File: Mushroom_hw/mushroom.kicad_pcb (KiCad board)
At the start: 2 copper layers, 49.2 x 83.8 mm, 129 parts, among them Q1 LED_RGB_WS2812B, Q2 LED_RGB, Q3 LED_RGB_WS2812B, Q4 LED_RGB, Q5 LED_RGB, Q6 LED_RGB_WS2812B, SW1 SWITCH_H

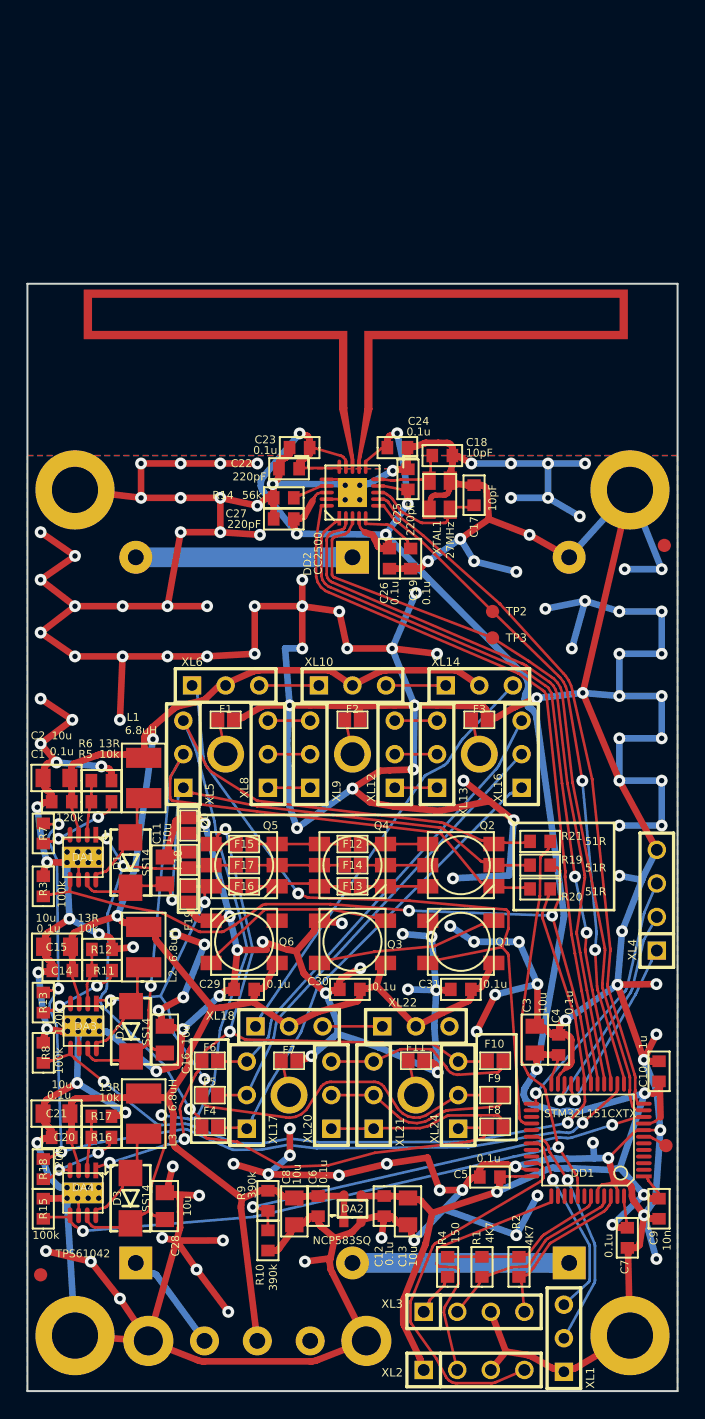
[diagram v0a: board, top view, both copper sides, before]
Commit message: + Component placement done
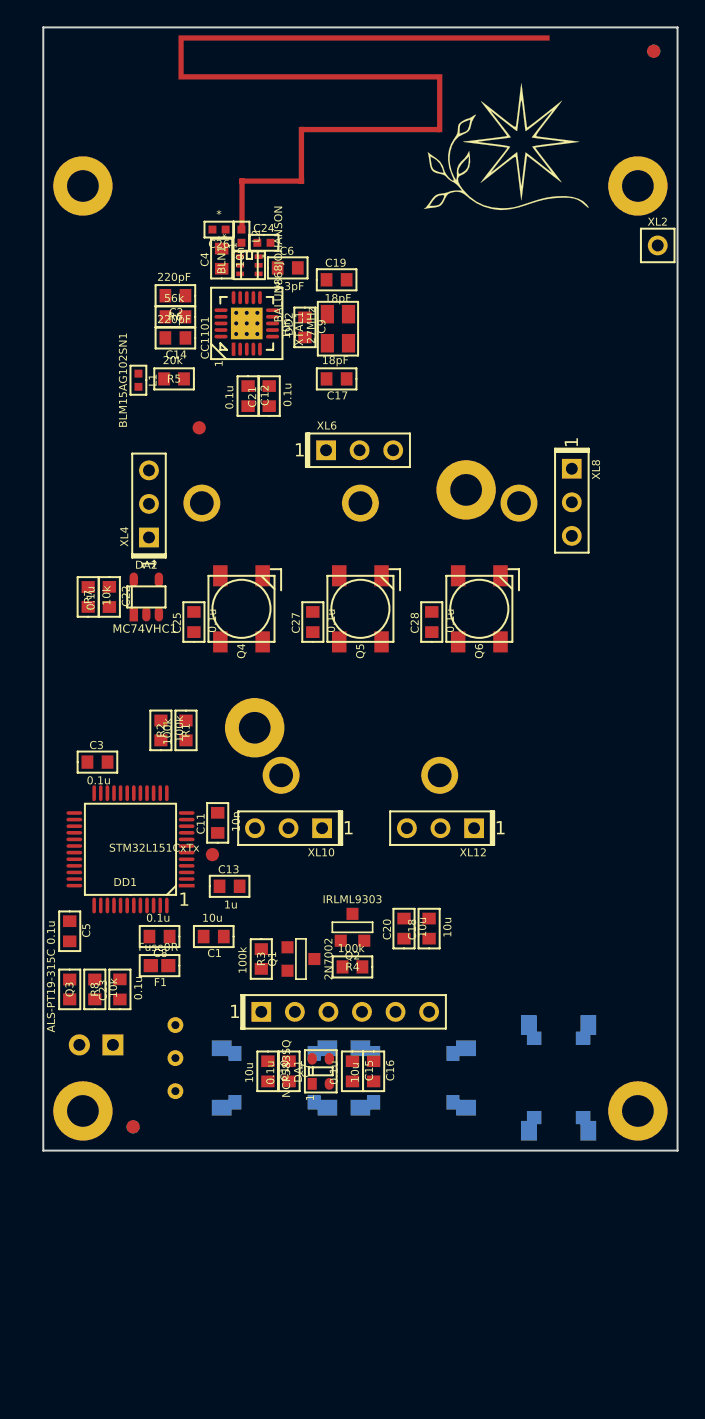
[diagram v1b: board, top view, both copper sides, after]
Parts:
- removed B1, B2, B3: BAT, BAT_AA
- removed C29, C30, C31: 0.1u, CAP_0603
- removed D1, D2, D3: SS14, DIODE_SMA_DO214AC
- removed DA3, DA4: TPS61042, DRB8
- removed F10, F11, F12, F13, F14, F15, F16, F17, F18, F19, F2, F20, F3, F4, F5, F6, F7, F8, F9: FUSE0R, SMD0603_FUSE
- removed L3: 6.8uH, IND_1210
- removed R10, R9: 390k, RES_0603
- removed R11, R16: 10k, RES_0603
- removed R12, R17: 13R, RES_0603
- removed R13, R18: 120k, RES_0603
- removed R14: 56k, RES_0603
- removed R15: 100k, RES_0603
- removed R19, R20, R21: 51R, RES_0603
- removed TP3: TESTPOINT, TESTPOINT_1MM
- removed XL14, XL16, XL17, XL18, XL20, XL21, XL22, XL24: CONN_3, SIL-3
- removed XL15, XL19, XL23: CONN_1, SIL1_ROUND_1MM8
- added BLN1: BALUN868JOHANSON, Radio:BALUN_JOHANSON868, F.Cu at (219.6, 130.0)
- added HOLE5: HOLE_METALLED, PCB:Hole2d4_out4d5mm, F.Cu at (249.0, 194.0)
- added HOLE6: HOLE_METALLED, PCB:Hole2d4_out4d5mm, F.Cu at (249.0, 124.0)
- added Logo1: Logo, Pictures:Ostranna_12d7_10d1, F.Cu at (239.0, 121.0)
- added RP3: REFPOINT, PCB:REF_POINT_1MM, B.Cu at (210.8, 195.2)
- added RP4: REFPOINT, PCB:REF_POINT_1MM, B.Cu at (250.2, 113.8)
- added SW2: BUTTON, BtnsSwitches:BTN_6x6_4x4, B.Cu at (243.0, 191.5)
- added SW3: BUTTON, BtnsSwitches:BTN_6x6_4x4, B.Cu at (221.5, 191.5)
- added SW4: BUTTON, BtnsSwitches:BTN_6x6_4x4, B.Cu at (232.0, 191.5)
- ANT1: value ANT_PCB_NOCNTR -> ANT_PCB_MONO; footprint ANT_FOLDED_DIPOLE2 -> Radio:ANT_868_ARMLETG
- C1, C20: value 0.1u -> 10u; footprint CAP_0603 -> Capacitors:CAP_0603
- C10: value 1u -> 10u; footprint CAP_0603 -> Capacitors:CAP_0603
- C11: value 10u -> 10n; footprint CAP_0805 -> Capacitors:CAP_0603
- C12, C23, C5, C7, C9: footprint CAP_0603 -> Capacitors:CAP_0603
- C13: value 10u -> 1u; footprint CAP_0805 -> Capacitors:CAP_0603
- C14: value 0.1u -> 220pF; footprint CAP_0603 -> Capacitors:CAP_0603
- C15, C21, C28, C3, C8: value 10u -> 0.1u; footprint CAP_0805 -> Capacitors:CAP_0603
- C16: footprint CAP_0805 -> Capacitors:CAP_0603
- C17: value 10pF -> 18pF; footprint CAP_0603 -> Capacitors:CAP_0603
- C18: value 10pF -> 10u; footprint CAP_0603 -> Capacitors:CAP_0603
- C19: value 0.1u -> 18pF; footprint CAP_0603 -> Capacitors:CAP_0603
- C2: value 10u -> 220pF; footprint CAP_0805 -> Capacitors:CAP_0603
- C22, C25, C27: value 220pF -> 0.1u; footprint CAP_0603 -> Capacitors:CAP_0603
- C24, C26: value 0.1u -> *; footprint CAP_0603 -> Capacitors:CAP_0402
- C4: value 0.1u -> 10n; footprint CAP_0603 -> Capacitors:CAP_0603
- C6: value 0.1u -> 3.3pF; footprint CAP_0603 -> Capacitors:CAP_0603
- DA1: value TPS61042 -> NCP583SQ; footprint DRB8 -> SOT:SC82AB
- DA2: value NCP583SQ -> MC74VHC1; footprint SC82AB -> SOT:SOT23-5
- DD1: value STM32L151CXTX -> STM32L151CxTx; footprint LQFP48 -> LQFP_TQFP:LQFP48
- DD2: value CC2500 -> CC1101; footprint QFN20 -> QFN_DFN:QFN20
- F1: value FUSE0R -> Fuse0R; footprint SMD0603_FUSE -> Resistors:RES_0603_FUSE
- HOLE1, HOLE2, HOLE3, HOLE4: footprint Hole3_5_out6mm -> PCB:Hole2d4_out4d5mm
- L1: value 6.8uH -> BLM15AG102SN1; footprint IND_1210 -> Inductors:IND_0402
- L2: value 6.8uH -> *; footprint IND_1210 -> Inductors:IND_0402
- Q1: value LED_RGB_WS2812B -> 2N7002; footprint LED_WS2812B -> SOT:SOT23-3
- Q2: value LED_RGB -> IRLML9303; footprint LED_HH5050_RGB -> SOT:SOT23-3
- Q3: value LED_RGB_WS2812B -> ALS-PT19-315C; footprint LED_WS2812B -> Resistors:RES_0603
- Q4, Q5: value LED_RGB -> LED_RGB_WS2812B; footprint LED_HH5050_RGB -> LEDs:LED_WS2812B
- Q6: footprint LED_WS2812B -> LEDs:LED_WS2812B
- R1, R2: value 4K7 -> 100k; footprint RES_0603 -> Resistors:RES_0603
- R3: footprint RES_0603 -> Resistors:RES_0603
- R4: value 150 -> 100k; footprint RES_0603 -> Resistors:RES_0603
- R5: value 10k -> 20k; footprint RES_0603 -> Resistors:RES_0603
- R6: value 13R -> 56k; footprint RES_0603 -> Resistors:RES_0603
- R7: value 120k -> 10k; footprint RES_0603 -> Resistors:RES_0603
- R8: value 100k -> 10k; footprint RES_0603 -> Resistors:RES_0603
- RP1, RP2: footprint REF_POINT_1MM -> PCB:REF_POINT_1MM
- SW1: value SWITCH_H -> SWITCH; footprint SWITCH_SS9 -> BtnsSwitches:SW_SS-1P2T
- TP1, TP2: footprint TESTPOINT_1MM -> PCB:TESTPOINT_1MM
- XL1: value CONN_3 -> CONN_6; footprint SIL-3 -> Connectors:PLS-6; moved to B.Cu
- XL10, XL12, XL6, XL8: footprint SIL-3 -> Connectors:PLS-3
- XL11, XL7: footprint SIL1_ROUND_1MM8 -> Connectors:SIL1_ROUND_1MM8
- XL13, XL5, XL9: value CONN_3 -> CONN_1; footprint SIL-3 -> Connectors:SIL1_ROUND_1MM8
- XL2: value ST_SWD -> CONN_1; footprint SIL-4 -> Connectors:PLS-1Rnd
- XL3: value CONN_4 -> CONN_2; footprint SIL-4 -> Connectors:W02_Pitch_2d54; moved to B.Cu
- XL4: value CONN_4 -> CONN_3; footprint SIL-4 -> Connectors:PLS-3
- XTAL1: footprint CRYSTAL_03225C4 -> Quartz:03225C4
- moved RP1 103.6 mm to (250.2, 113.8)
- moved XL2 86.2 mm to (250.5, 128.5)
- moved C9 71.9 mm to (223.8, 134.7)
- moved C6 71.0 mm to (222.5, 130.2), turned to 0 degrees
- moved C4 64.7 mm to (217.5, 129.5)
- moved C12 62.2 mm to (219.5, 139.9)
- moved RP2 59.6 mm to (210.8, 195.2)
- moved C21 56.6 mm to (221.1, 139.9), turned to 90 degrees
- moved L2 54.3 mm to (219.0, 127.8), turned to 270 degrees
- moved HOLE2 54.1 mm to (220.0, 165.0)
- moved DA2 48.9 mm to (211.8, 155.1), turned to 0 degrees
- moved R2 48.8 mm to (212.9, 165.2)
- moved C14 48.6 mm to (214.0, 135.5)
- moved C28 48.6 mm to (233.4, 157.0)
- moved HOLE4 47.4 mm to (207.0, 124.0)
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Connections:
- ANT1 pad 1: /Ant -> /ANT2
- C1 pad 1: +BATT -> GND
- C1 pad 2: GND -> +3.3V
- C10 pad 1: +3.3V -> +BATT
- C11 pad 1: /RED_P -> +3.3V
- C12 pad 1: +3.3V -> VCC
- C14 pad 1: +BATT -> VCC
- C15 pad 1: +BATT -> +3.3V
- C16 pad 1: /GREEN_P -> +3.3V
- C18 pad 1: N-000005 -> GND
- C18 pad 2: GND -> PwrUnst
- C19 pad 1: N-0000010 -> Net-(C19-Pad1)
- C2 pad 1: +BATT -> VCC
- C20 pad 1: +BATT -> GND
- C20 pad 2: GND -> PwrUnst
- C21 pad 1: +BATT -> GND
- C21 pad 2: GND -> Net-(C21-Pad2)
- C22 pad 1: +3.3V -> PwrUnst
- C23 pad 1: +3.3V -> /ADC_LUM
- C24 pad 1: +3.3V -> /ANT1
- C25 pad 1: +3.3V -> PwrUnst
- C26 pad 1: +3.3V -> /ANT2
- C27 pad 1: +3.3V -> PwrUnst
- C28 pad 1: /BLUE_P -> PwrUnst
- C4 pad 1: +3.3V -> VCC
- C6 pad 1: +BATT -> VCC
- C7 pad 1: +3.3V -> +BATT
- C8 pad 1: +BATT -> +3.3V
- C9 pad 1: +3.3V -> VCC
- DA1 pad 1: /RED_N -> +BATT
- DA1 pad 2: N-000007 -> GND
- DA1 pad 3: +BATT -> +3.3V
- DA1 pad 4: N-000006 -> +BATT
- DA2 pad 1: +BATT -> Net-(DA2-Pad1)
- DA2 pad 2: GND -> /WS_CTRL
- DA2 pad 3: +3.3V -> GND
- DA2 pad 4: +BATT -> /DIN0
- DD1 pad 10: N-000008 -> /BTN1
- DD1 pad 11: /CC_GDO2 -> /BTN2
- DD1 pad 12: /CC_CS -> /ADC_BATTERY
- DD1 pad 14: /BRIGHTNESS -> /CC_CS
- DD1 pad 18: /RED_PWM -> /ADC_LUM
- DD1 pad 19: /GREEN_PWM -> /MEAS_LUM
- DD1 pad 21: N-0000032 -> (no net)
- DD1 pad 22: N-0000033 -> (no net)
- DD1 pad 25: N-0000031 -> (no net)
- DD1 pad 27: (no net) -> /PWR_EN
- DD1 pad 28: /DIN0 -> /WS_CTRL
- DD1 pad 29: (no net) -> /BTN3
- DD1 pad 41: /BLUE_PWM -> (no net)
- DD1 pad 43: /PeriphPwr -> /NO_RADIO
- DD1 pad 45: /P_SCL -> (no net)
- DD1 pad 46: /P_SDA -> (no net)
- DD2 pad 10: N-000005 -> Net-(C19-Pad1)
- DD2 pad 11: +3.3V -> VCC
- DD2 pad 12: /Ant -> /RF1
- DD2 pad 13: /Ant -> /RF2
- DD2 pad 14: +3.3V -> VCC
- DD2 pad 15: +3.3V -> VCC
- DD2 pad 17: N-0000013 -> Net-(DD2-Pad17)
- DD2 pad 18: +3.3V -> VCC
- DD2 pad 3: /CC_GDO2 -> (no net)
- DD2 pad 4: +3.3V -> VCC
- DD2 pad 5: N-0000010 -> Net-(C21-Pad2)
- DD2 pad 9: +3.3V -> VCC
- F1 pad 1: GND -> +3.3V
- F1 pad 2: N-0000070 -> /NO_RADIO
- L1 pad 1: N-0000017 -> VCC
- L1 pad 2: +BATT -> +3.3V
- L2 pad 1: N-0000016 -> /ANT2
- L2 pad 2: +BATT -> /ANT1
- Q1 pad 1: +BATT -> /PWR_EN
- Q1 pad 2: N-0000059 -> GND
- Q1 pad 3: GND -> Net-(Q1-Pad3)
- Q3 pad 1: +BATT -> +3.3V
- Q3 pad 2: N-0000058 -> /ADC_LUM
- Q6 pad 1: +BATT -> PwrUnst
- Q6 pad 4: N-0000058 -> Net-(Q5-Pad2)
- R1 pad 1: /P_SCL -> PwrUnst
- R1 pad 2: /PeriphPwr -> /ADC_BATTERY
- R2 pad 1: /P_SDA -> /ADC_BATTERY
- R2 pad 2: /PeriphPwr -> GND
- R3 pad 1: /RED_PWM -> /PWR_EN
- R4 pad 1: /PeriphPwr1 -> +BATT
- R4 pad 2: /PeriphPwr -> Net-(Q1-Pad3)
- R5 pad 1: N-000007 -> /CC_CS
- R5 pad 2: N-000006 -> VCC
- R6 pad 1: N-000007 -> Net-(DD2-Pad17)
- R7 pad 1: N-000006 -> Net-(DA2-Pad1)
- R7 pad 2: /BRIGHTNESS -> PwrUnst
- R8 pad 1: /GREEN_PWM -> /ADC_LUM
- R8 pad 2: GND -> /MEAS_LUM
- SW1 pad 1: /BAT_IN -> +BATT
- SW1 pad 2: +BATT -> /BAT_IN
- XL1 pad 1: GND -> +3.3V
- XL1 pad 2: /UART_TX -> /SWCLK
- XL1 pad 3: /UART_RX -> GND
- XL10 pad 1: /DIN1 -> /DIN3
- XL10 pad 2: +BATT -> PwrUnst
- XL10 pad 3: /DIN2 -> /DIN4
- XL11 pad 1: N-0000071 -> GND
- XL12 pad 1: N-0000022 -> /DIN4
- XL12 pad 2: N-0000021 -> PwrUnst
- XL12 pad 3: N-0000020 -> (no net)
- XL13 pad 1: N-0000022 -> GND
- XL2 pad 1: +3.3V -> GND
- XL3 pad 1: /PeriphPwr1 -> /BAT_IN
- XL3 pad 2: /P_SCL -> GND
- XL4 pad 1: N-0000032 -> /DIN0
- XL4 pad 2: N-0000033 -> PwrUnst
- XL4 pad 3: N-0000031 -> /DIN1
- XL5 pad 1: /RED_P -> GND
- XL6 pad 1: /DIN0 -> /DIN1
- XL6 pad 2: +BATT -> PwrUnst
- XL6 pad 3: /DIN1 -> /DIN2
- XL7 pad 1: N-0000070 -> GND
- XL8 pad 1: N-0000028 -> /DIN2
- XL8 pad 2: N-0000027 -> PwrUnst
- XL8 pad 3: N-0000026 -> /DIN3
- XL9 pad 1: N-0000028 -> GND
- XTAL1 pad 2: N-000005 -> Net-(C19-Pad1)
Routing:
- net GND: track 812.5 -> 0.00 mm, vias 151 -> 0
- net +3.3V: track 177.8 -> 0.00 mm, vias 10 -> 0
- net +BATT: track 159.2 -> 0.00 mm, vias 2 -> 0
- net /BLUE_P: track 78.3 -> 0.00 mm, vias 1 -> 0
- net /BRIGHTNESS: track 73.8 -> 0.00 mm, vias 4 -> 0
- net /BLUE_PWM: track 68.9 -> 0.00 mm, vias 2 -> 0
- net /GREEN_P: track 62.2 -> 0.00 mm, vias 1 -> 0
- net /GREEN_PWM: track 61.7 -> 0.00 mm, vias 2 -> 0
- net /RED_N: track 60.8 -> 0.00 mm, vias 3 -> 0
- net /RED_PWM: track 58.2 -> 0.00 mm, vias 2 -> 0
- net /BLUE_N: track 58.1 -> 0.00 mm, vias 4 -> 0
- net /CC_GDO2: track 58.0 -> 0.00 mm
- net /DIN0: track 57.0 -> 0.00 mm, vias 1 -> 0
- net /CC_MOSI: track 55.4 -> 0.00 mm
- net /CC_MISO: track 55.0 -> 0.00 mm
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- removed copper zone on B.Cu, net GND
- removed copper zone on F.Cu, net GND
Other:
- board size 49.2 x 83.8 mm -> 48 x 85 mm
